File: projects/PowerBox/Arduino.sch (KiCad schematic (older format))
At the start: 63 parts, among them CON3 USB-MINI-B-Vert, IC3 LM358, P10 Analog, P11 CONN_10, P12 CONN_8, P13 CONN_8, P14 CONN_6, P15 Digital, P7 CONN_3X2, P8 Serial, P9 I2C, Q4 DMG3415U, Q5 DMG3415U, U4 INA219, U5 AP7333, U6 ATMEGA32U4, X1 16MHz

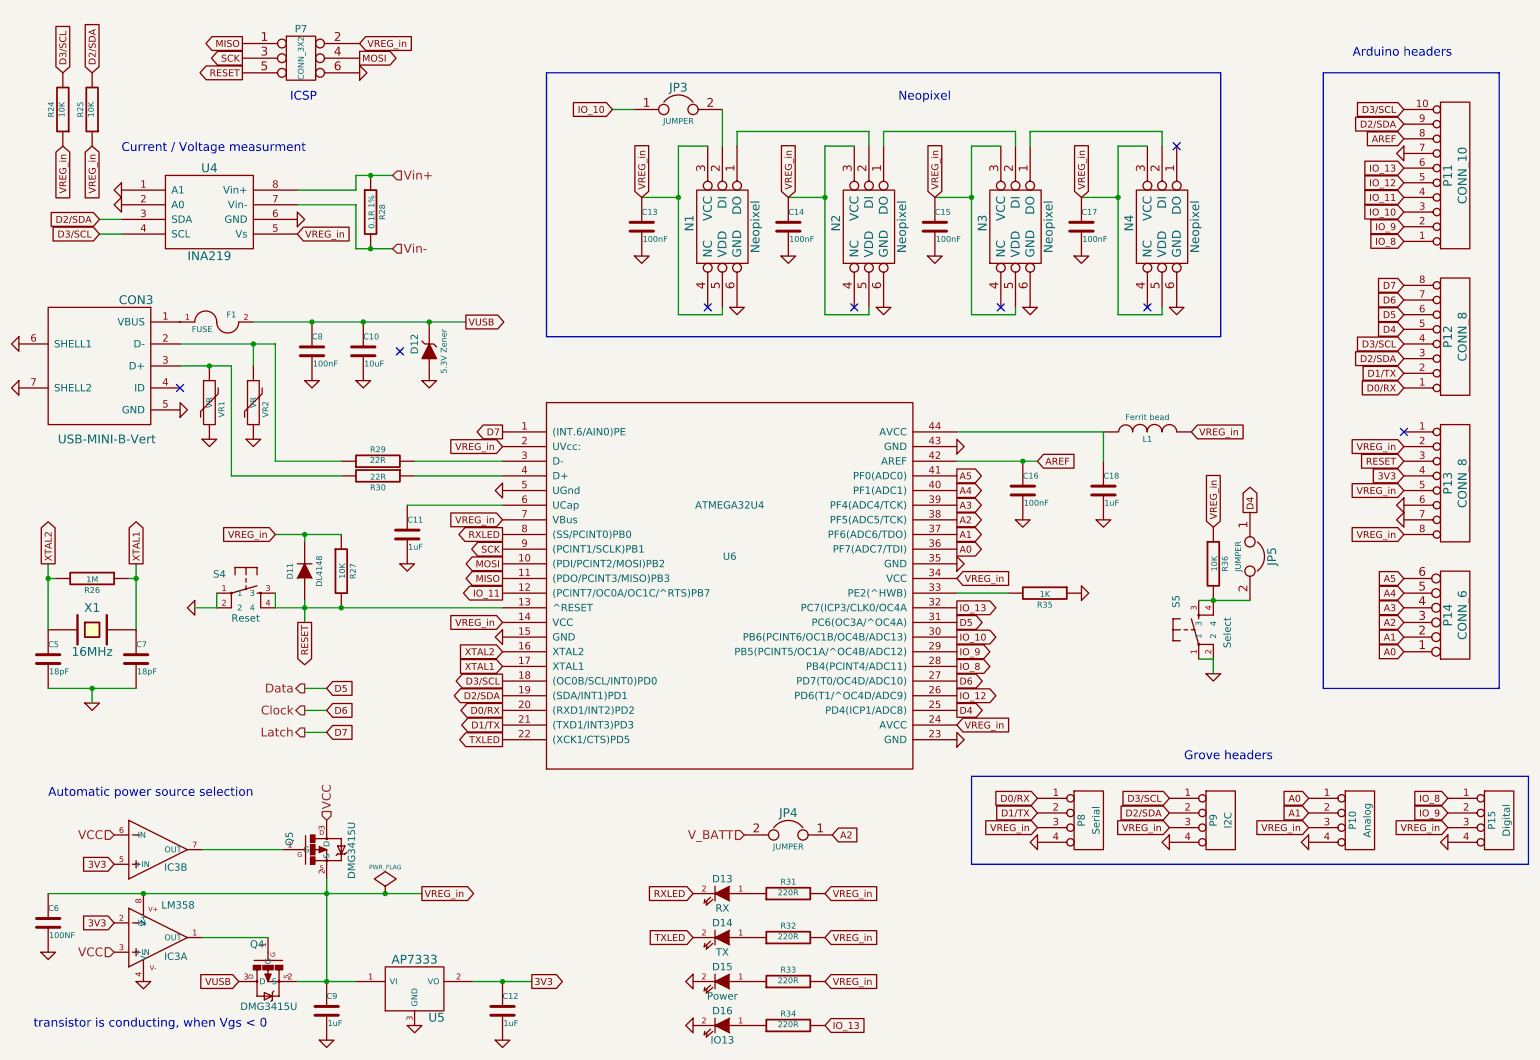
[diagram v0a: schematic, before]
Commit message: layout in progress
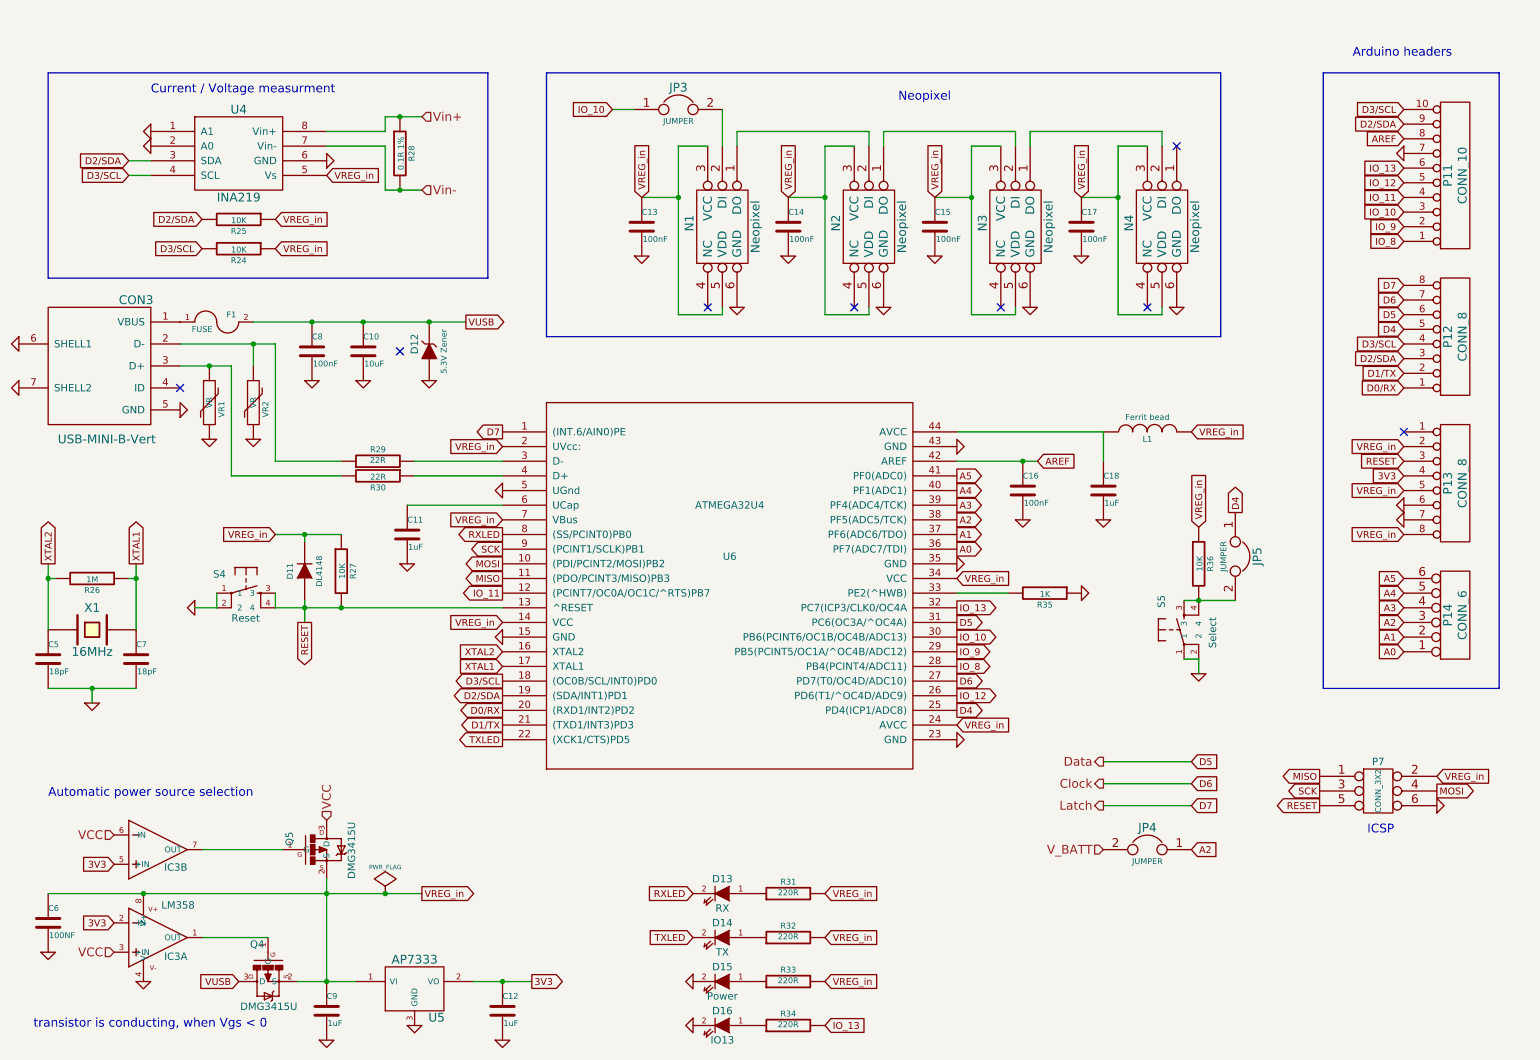
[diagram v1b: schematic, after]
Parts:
- removed P10: Analog, frep:grove_con_straight, symbol CONN_4
- removed P15: Digital, frep:grove_con_straight, symbol CONN_4
- removed P8: Serial, frep:grove_con_straight, symbol CONN_4
- removed P9: I2C, frep:grove_con_straight, symbol CONN_4
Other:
- note removed: "Grove headers"
- moved on the sheet: JP4, JP5, P7, R24, R25, R28, R36, S5, U4
